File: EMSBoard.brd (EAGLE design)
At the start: 66 x 25.4 mm, 5 parts, among them IC2 BLUE_PILL, J1 B2B-XH-A__LF__SN_

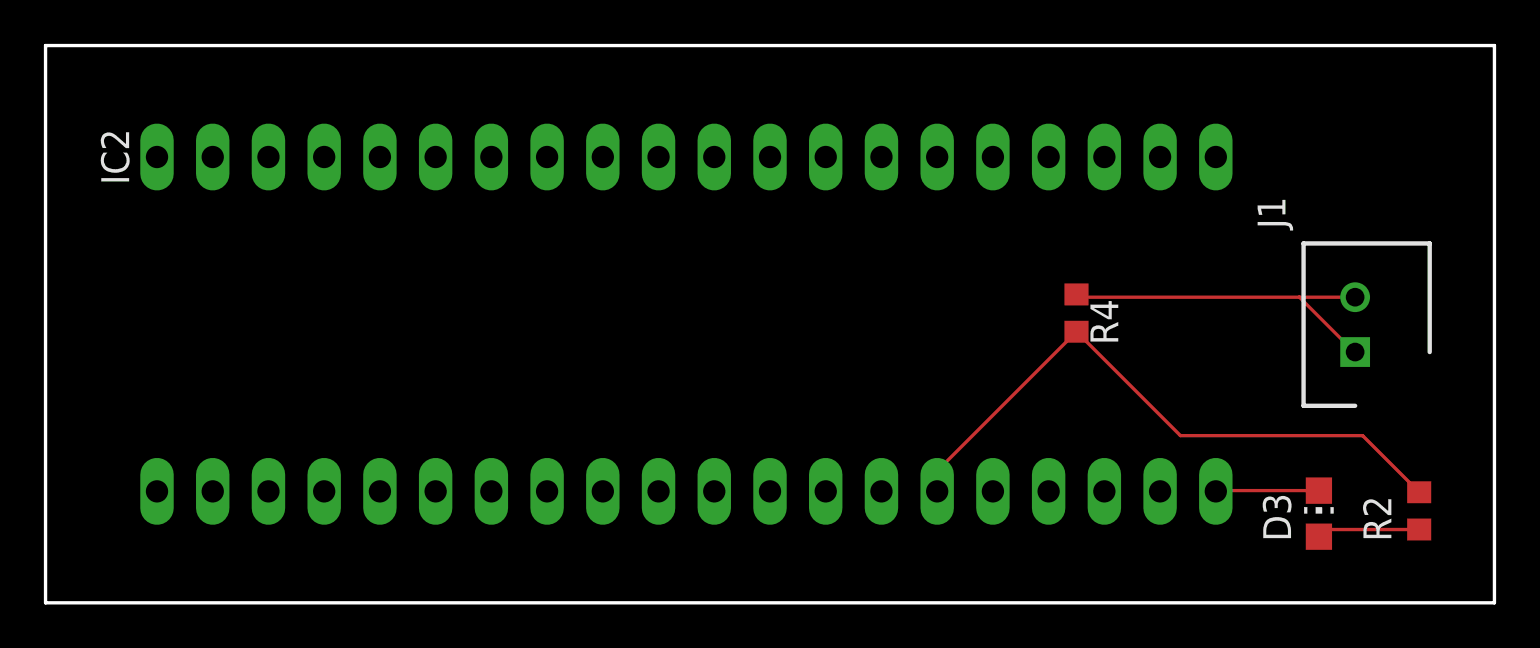
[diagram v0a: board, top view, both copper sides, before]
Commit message: Resolve Conflicts
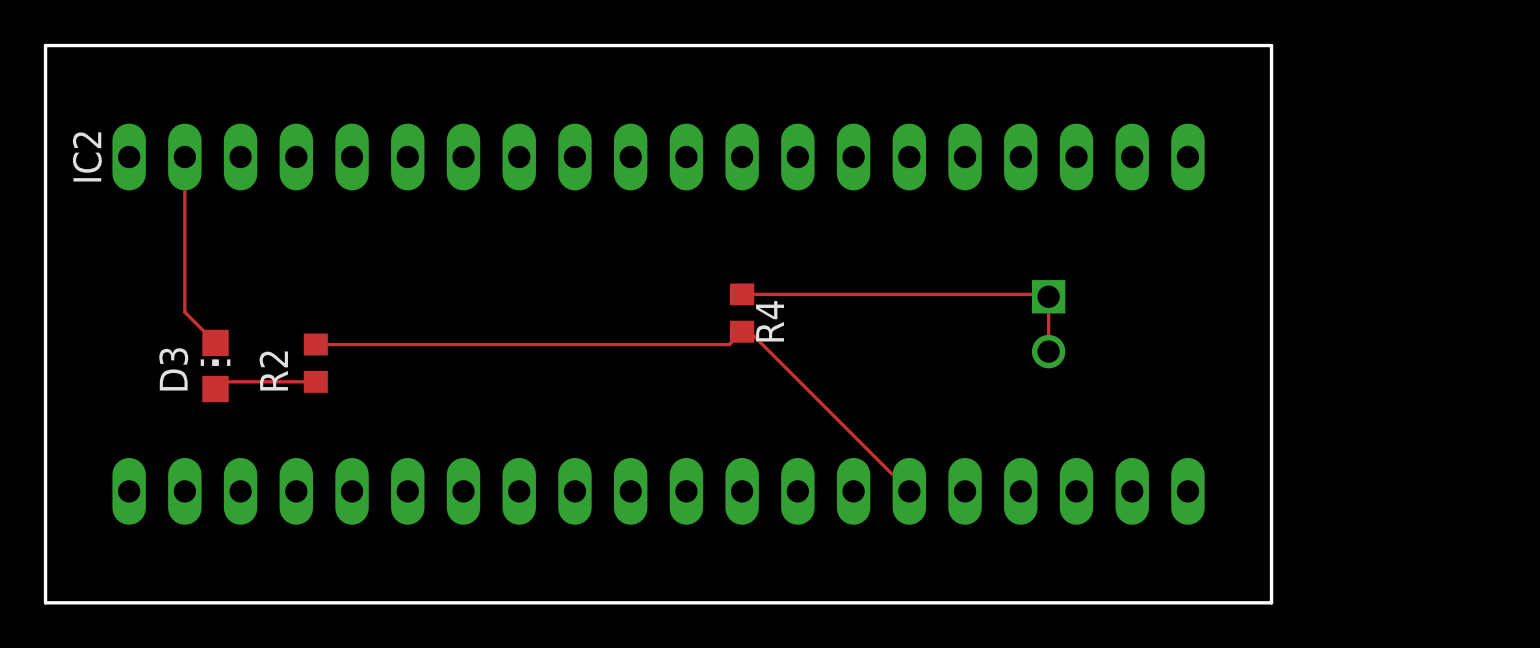
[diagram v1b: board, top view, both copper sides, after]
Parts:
- J1: value B2B-XH-A__LF__SN_ -> (none); device SamacSys_Parts:SHDR2W64P0X250_1X2_740X575X700 -> jst-xh:S2B-XH-A
- moved D3 50.7 mm to (7.75, 10.8)
- moved R2 50.7 mm to (12.3, 10.9)
- moved R4 15.2 mm to (31.8, 13.2)
- moved J1 14.0 mm to (45.7, 12.7), flipped to the bottom
- moved IC2 1.27 mm to (14.0, 12.7)
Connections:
- net GND: now also IC2.P$39; no longer IC2.P$20
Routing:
- net GND: track 4.71 -> 9.05 mm
- net N$3: track 28.6 -> 30.3 mm
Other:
- board size 66 x 25.4 mm -> 55.9 x 25.4 mm
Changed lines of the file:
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@@
 <board>
 <plain>
-<wire x1="0" y1="0" x2="66.04" y2="0" width="0.1524" layer="20"/>
-<wire x1="66.04" y1="25.4" x2="0" y2="25.4" width="0.1524" layer="20"/>
 <wire x1="0" y1="25.4" x2="0" y2="0" width="0.1524" layer="20"/>
-<wire x1="66.04" y1="0" x2="66.04" y2="25.4" width="0.1524" layer="20"/>
+<wire x1="0" y1="25.4" x2="55.88" y2="25.4" width="0.1524" layer="20"/>
+<wire x1="55.88" y1="25.4" x2="55.88" y2="0" width="0.1524" layer="20"/>
+<wire x1="55.88" y1="0" x2="0" y2="0" width="0.1524" layer="20"/>
 </plain>
 <attributes>
@@
 </autorouter>
 <elements>
-<element name="D3" library="led" library_urn="urn:adsk.eagle:library:259" package="CHIP-LED0805" package3d_urn="urn:adsk.eagle:package:15818/2" value="" x="58.039" y="4.064" smashed="yes">
-<attribute name="NAME" x="56.769" y="2.794" size="1.27" layer="25" rot="R90"/>
-<attribute name="POPULARITY" value="68" x="99.949" y="-55.626" size="1.778" layer="27" display="off"/>
-<attribute name="VALUE" x="60.579" y="2.794" size="1.27" layer="27" rot="R90"/>
-</element>
-<element name="IC2" library="stm32_mcu" package="BLUE_PILL" value="BLUE_PILL" x="15.24" y="12.7" smashed="yes" rot="R90">
-<attribute name="NAME" x="3.81" y="19.05" size="1.27" layer="25" rot="R90"/>
-</element>
-<element name="J1" library="SamacSys_Parts" package="SHDR2W64P0X250_1X2_740X575X700" value="B2B-XH-A__LF__SN_" x="59.69" y="11.43" smashed="yes" rot="R90">
-<attribute name="ARROW_PART_NUMBER" value="" x="120.65" y="34.29" size="1.778" layer="27" rot="R90" display="off"/>
-<attribute name="ARROW_PRICE-STOCK" value="" x="120.65" y="34.29" size="1.778" layer="27" rot="R90" display="off"/>
-<attribute name="DESCRIPTION" value="JST (JAPAN SOLDERLESS TERMINALS) - B2B-XH-A (LF)(SN) - HEADER, VERTICAL, 2WAY" x="120.65" y="34.29" size="1.778" layer="27" rot="R90" display="off"/>
-<attribute name="HEIGHT" value="7mm" x="120.65" y="34.29" size="1.778" layer="27" rot="R90" display="off"/>
-<attribute name="MANUFACTURER_NAME" value="JST (JAPAN SOLDERLESS TERMINALS)" x="120.65" y="34.29" size="1.778" layer="27" rot="R90" display="off"/>
-<attribute name="MANUFACTURER_PART_NUMBER" value="B2B-XH-A (LF)(SN)" x="120.65" y="34.29" size="1.778" layer="27" rot="R90" display="off"/>
-<attribute name="MOUSER_PART_NUMBER" value="" x="120.65" y="34.29" size="1.778" layer="27" rot="R90" display="off"/>
-<attribute name="MOUSER_PRICE-STOCK" value="" x="120.65" y="34.29" size="1.778" layer="27" rot="R90" display="off"/>
-<attribute name="MOUSER_TESTING_PART_NUMBER" value="" x="120.65" y="34.29" size="1.778" layer="27" rot="R90" display="off"/>
-<attribute name="MOUSER_TESTING_PRICE-STOCK" value="" x="120.65" y="34.29" size="1.778" layer="27" rot="R90" display="off"/>
-<attribute name="NAME" x="55.88" y="17.78" size="1.27" layer="25" rot="R90" align="center"/>
-</element>
-<element name="R2" library="rcl" library_urn="urn:adsk.eagle:library:334" package="R0603" package3d_urn="urn:adsk.eagle:package:23555/3" value="1k" x="62.611" y="4.191" smashed="yes" rot="R90">
-<attribute name="NAME" x="61.341" y="2.794" size="1.27" layer="25" rot="R90"/>
-<attribute name="POPULARITY" value="70" x="122.301" y="43.561" size="1.778" layer="27" rot="R90" display="off"/>
-<attribute name="SPICEPREFIX" value="R" x="122.301" y="43.561" size="1.778" layer="27" rot="R90" display="off"/>
-</element>
-<element name="R4" library="rcl" library_urn="urn:adsk.eagle:library:334" package="R0603" package3d_urn="urn:adsk.eagle:package:23555/3" value="100" x="46.99" y="13.208" smashed="yes" rot="R270">
-<attribute name="NAME" x="47.625" y="13.843" size="1.27" layer="25" rot="R270"/>
-<attribute name="POPULARITY" value="70" x="-12.7" y="-22.352" size="1.778" layer="27" rot="R270" display="off"/>
-<attribute name="SPICEPREFIX" value="R" x="-12.7" y="-22.352" size="1.778" layer="27" rot="R270" display="off"/>
-<attribute name="VALUE" x="45.085" y="13.843" size="1.27" layer="27" rot="R270"/>
+<element name="D3" library="led" library_urn="urn:adsk.eagle:library:259" package="CHIP-LED0805" package3d_urn="urn:adsk.eagle:package:15818/2" value="" x="7.747" y="10.795" smashed="yes">
+<attribute name="NAME" x="6.477" y="9.525" size="1.27" layer="25" rot="R90"/>
+<attribute name="POPULARITY" value="68" x="49.657" y="-48.895" size="1.778" layer="27" display="off"/>
+<attribute name="VALUE" x="10.287" y="9.525" size="1.27" layer="27" rot="R90"/>
+</element>
+<element name="IC2" library="stm32_mcu" package="BLUE_PILL" value="BLUE_PILL" x="13.97" y="12.7" smashed="yes" rot="R90">
+<attribute name="NAME" x="2.54" y="19.05" size="1.27" layer="25" rot="R90"/>
+</element>
+<element name="J1" library="jst-xh" package="S2B-XH-A" value="" x="45.72" y="12.7" smashed="yes" rot="MR90">
+<attribute name="NAME" x="49.53" y="19.05" size="1.27" layer="26" rot="MR90" align="center"/>
+</element>
+<element name="R2" library="rcl" library_urn="urn:adsk.eagle:library:334" package="R0603" package3d_urn="urn:adsk.eagle:package:23555/3" value="1k" x="12.319" y="10.922" smashed="yes" rot="R90">
+<attribute name="NAME" x="11.049" y="9.525" size="1.27" layer="25" rot="R90"/>
+<attribute name="POPULARITY" value="70" x="72.009" y="50.292" size="1.778" layer="27" rot="R90" display="off"/>
+<attribute name="SPICEPREFIX" value="R" x="72.009" y="50.292" size="1.778" layer="27" rot="R90" display="off"/>
+</element>
+<element name="R4" library="rcl" library_urn="urn:adsk.eagle:library:334" package="R0603" package3d_urn="urn:adsk.eagle:package:23555/3" value="100" x="31.75" y="13.208" smashed="yes" rot="R270">
+<attribute name="NAME" x="32.385" y="13.843" size="1.27" layer="25" rot="R270"/>
+<attribute name="POPULARITY" value="70" x="-27.94" y="-22.352" size="1.778" layer="27" rot="R270" display="off"/>
+<attribute name="SPICEPREFIX" value="R" x="-27.94" y="-22.352" size="1.778" layer="27" rot="R270" display="off"/>
+<attribute name="VALUE" x="29.845" y="13.843" size="1.27" layer="27" rot="R270"/>
 </element>
 </elements>
@@
 <contactref element="D3" pad="A"/>
 <contactref element="R2" pad="1"/>
-<wire x1="62.611" y1="3.341" x2="58.366" y2="3.341" width="0.1524" layer="1"/>
-<wire x1="58.366" y1="3.341" x2="58.039" y2="3.014" width="0.1524" layer="1"/>
+<wire x1="12.319" y1="10.072" x2="8.074" y2="10.072" width="0.1524" layer="1"/>
+<wire x1="8.074" y1="10.072" x2="7.747" y2="9.745" width="0.1524" layer="1"/>
 </signal>
 <signal name="N$2">
@@
 <contactref element="R4" pad="1"/>
 <contactref element="J1" pad="1"/>
-<wire x1="59.69" y1="13.93" x2="57.15" y2="13.93" width="0.1524" layer="1"/>
-<wire x1="57.15" y1="13.93" x2="47.118" y2="13.93" width="0.1524" layer="1"/>
-<wire x1="47.118" y1="13.93" x2="46.99" y2="14.058" width="0.1524" layer="1"/>
-<wire x1="59.69" y1="11.43" x2="59.65" y2="11.43" width="0.1524" layer="1"/>
-<wire x1="59.65" y1="11.43" x2="57.15" y2="13.93" width="0.1524" layer="1"/>
+<wire x1="45.72" y1="11.45" x2="45.72" y2="13.95" width="0.1524" layer="1"/>
+<wire x1="45.72" y1="13.95" x2="45.612" y2="14.058" width="0.1524" layer="1"/>
+<wire x1="45.612" y1="14.058" x2="31.75" y2="14.058" width="0.1524" layer="1"/>
 </signal>
 <signal name="N$3">
@@
 <contactref element="R4" pad="2"/>
 <contactref element="R2" pad="2"/>
-<wire x1="46.99" y1="12.358" x2="40.64" y2="6.008" width="0.1524" layer="1"/>
-<wire x1="40.64" y1="6.008" x2="40.64" y2="5.08" width="0.1524" layer="1"/>
-<wire x1="46.99" y1="12.358" x2="51.728" y2="7.62" width="0.1524" layer="1"/>
-<wire x1="60.032" y1="7.62" x2="62.611" y2="5.041" width="0.1524" layer="1"/>
-<wire x1="51.728" y1="7.62" x2="60.032" y2="7.62" width="0.1524" layer="1"/>
+<wire x1="12.319" y1="11.772" x2="31.164" y2="11.772" width="0.1524" layer="1"/>
+<wire x1="31.164" y1="11.772" x2="31.75" y2="12.358" width="0.1524" layer="1"/>
+<wire x1="31.75" y1="12.358" x2="32.092" y2="12.358" width="0.1524" layer="1"/>
+<wire x1="32.092" y1="12.358" x2="39.37" y2="5.08" width="0.1524" layer="1"/>
 </signal>
 <signal name="GND">
-<contactref element="IC2" pad="P$20"/>
 <contactref element="D3" pad="C"/>
-<wire x1="53.34" y1="5.08" x2="53.374" y2="5.114" width="0.1524" layer="1"/>
-<wire x1="53.374" y1="5.114" x2="58.039" y2="5.114" width="0.1524" layer="1"/>
+<contactref element="IC2" pad="P$39"/>
+<wire x1="7.747" y1="11.845" x2="6.35" y2="13.242" width="0.1524" layer="1"/>
+<wire x1="6.35" y1="13.242" x2="6.35" y2="20.32" width="0.1524" layer="1"/>
 </signal>
 </signals>
